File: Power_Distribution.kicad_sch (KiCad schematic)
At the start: 37 parts, among them U4 LT1963AEST-3.3#TRPBF, U5 TPS2115ADRBR, U6 TPS5405DR

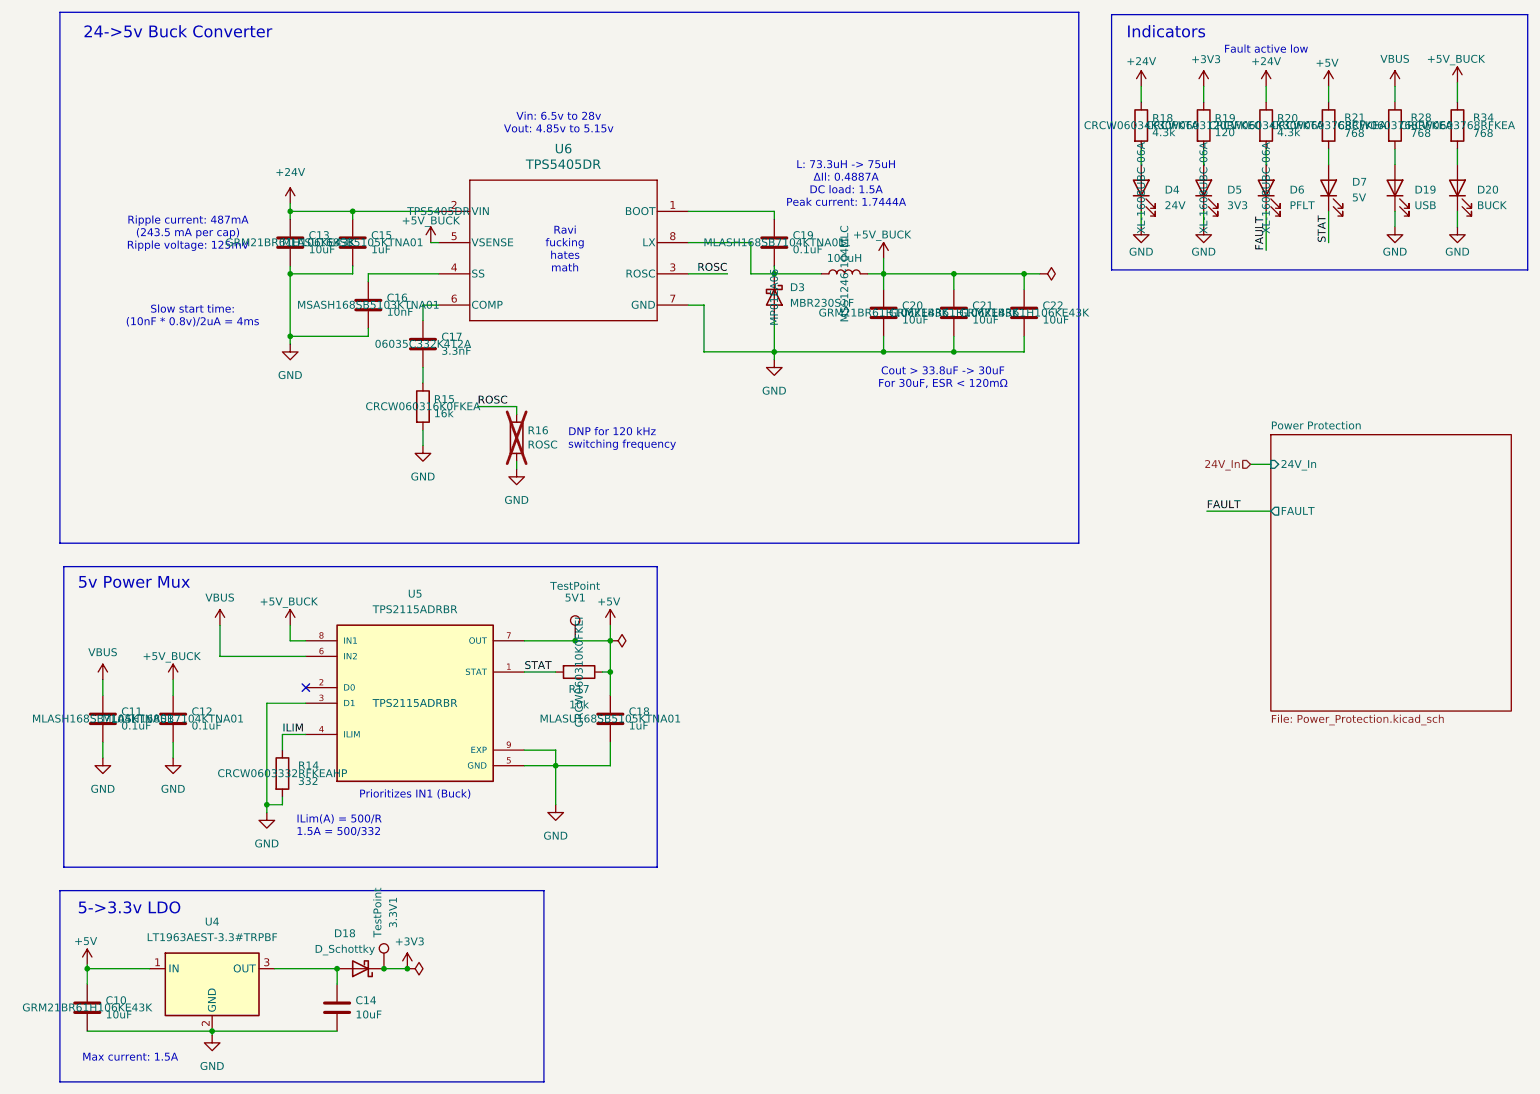
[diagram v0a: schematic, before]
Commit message: comp spares with fixed ldo diode
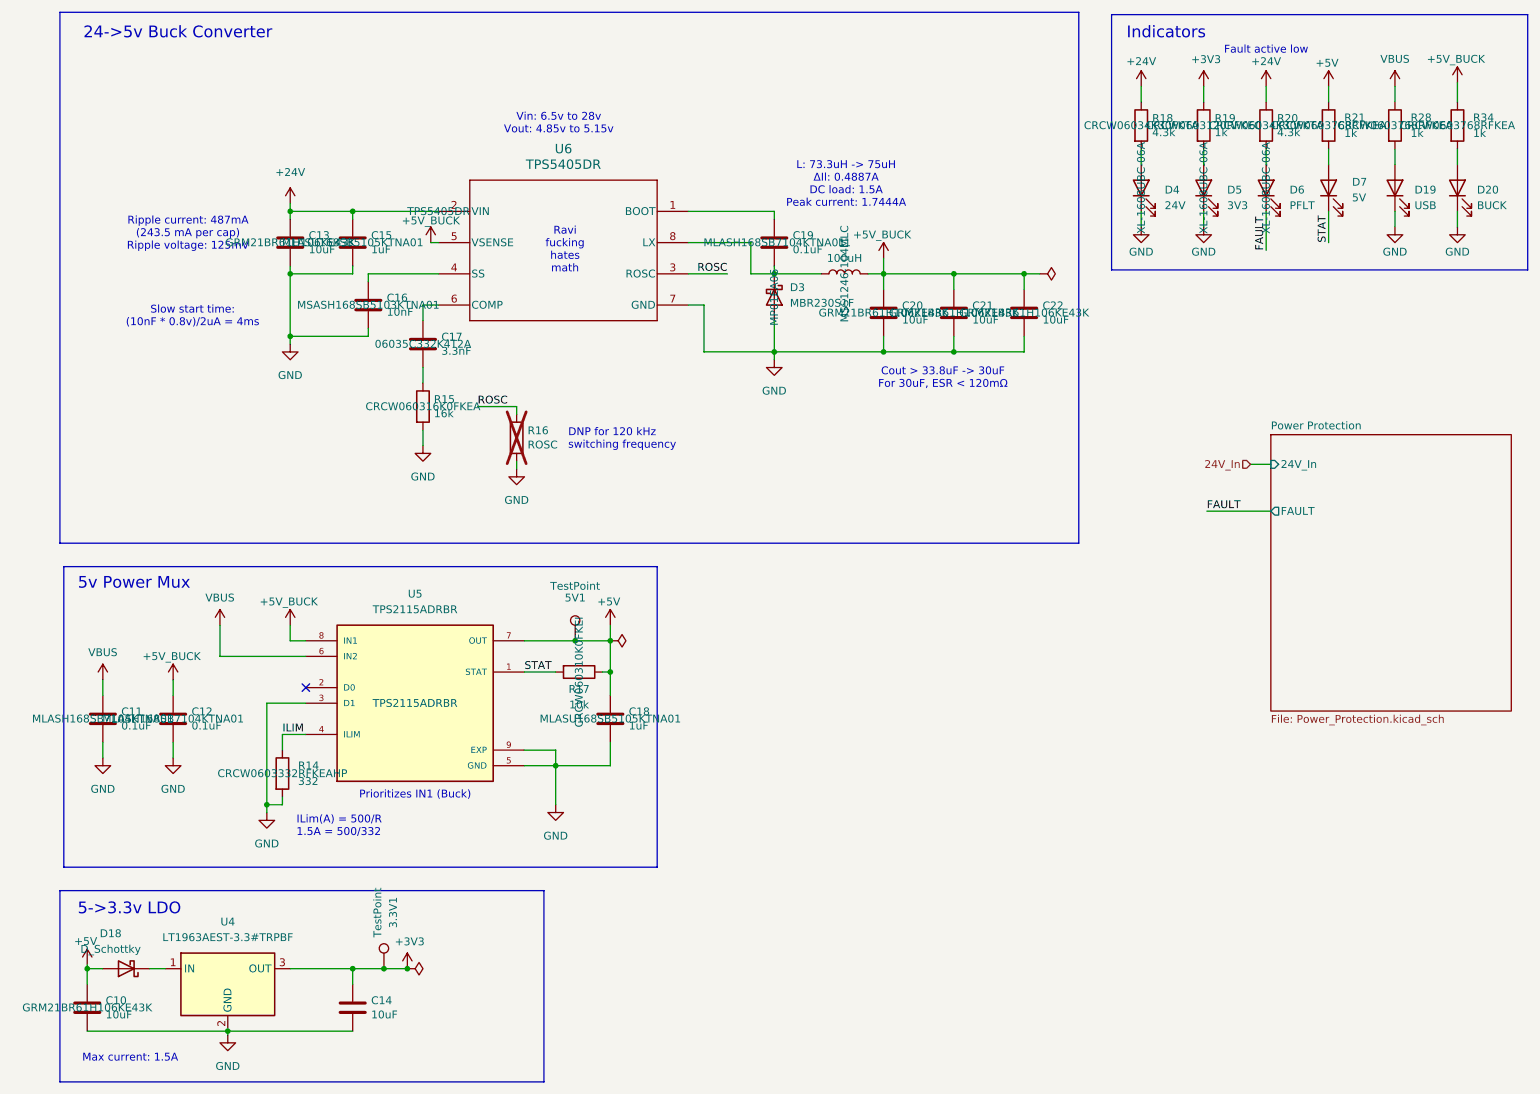
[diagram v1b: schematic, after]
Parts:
- R19: value 120 -> 1k
- R21, R28, R34: value 768 -> 1k
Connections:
- net +3V3: now also C14.1, U4.3 (OUT); no longer D18.1 (K)
- net +5V: now also D18.2 (A); no longer U4.1 (IN)
- new net: D18.1 (K), U4.1 (IN)
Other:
- moved on the sheet: C14, D18, U4
